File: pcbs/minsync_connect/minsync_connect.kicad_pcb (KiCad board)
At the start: 2 copper layers, 17.4 x 14 mm, 2 parts, among them J1 Left, J2 Right

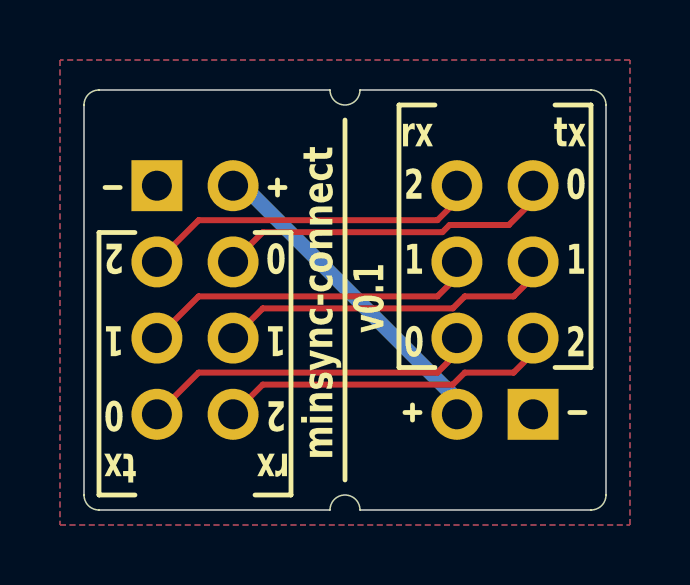
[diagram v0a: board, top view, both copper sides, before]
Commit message: Order minsync
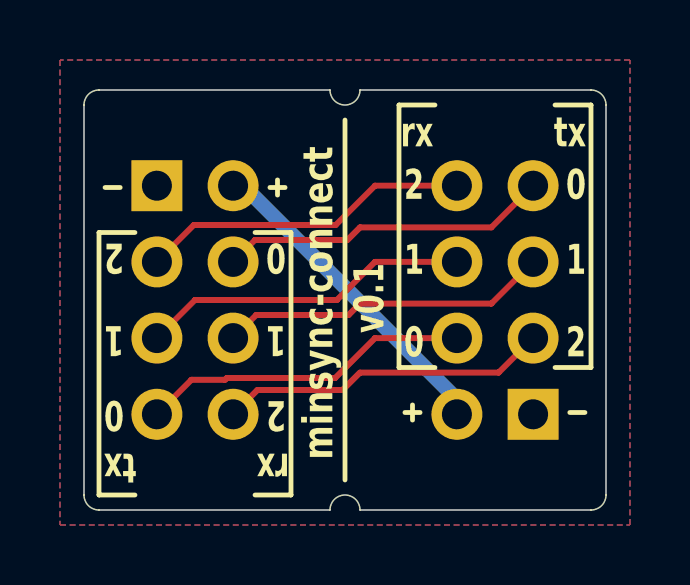
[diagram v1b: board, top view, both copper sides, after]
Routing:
- net /L_TX2: track 11.6 -> 11.1 mm
- net /L_TX0: track 11.6 -> 11.1 mm
- net /L_RX2: track 11.6 -> 11.1 mm
- net /L_RX0: track 11.6 -> 11.1 mm
- net /L_TX1: track 11.6 -> 11.1 mm
- net /L_RX1: track 11.6 -> 11.1 mm
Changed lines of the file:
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@@
 	)
 	(segment
-		(start 152.26 42.82)
-		(end 158.593654 42.82)
+		(start 155.5 42.42)
+		(end 160.12 42.42)
+		(width 0.2)
+		(layer "F.Cu")
+		(net 1)
+	)
+	(segment
+		(start 160.12 42.42)
+		(end 161.27 41.27)
+		(width 0.2)
+		(layer "F.Cu")
+		(net 1)
+	)
+	(segment
+		(start 154.92 43)
+		(end 155.5 42.42)
 		(width 0.2)
 		(layer "F.Cu")
@@
 	(segment
 		(start 151.27 43.81)
-		(end 152.26 42.82)
-		(width 0.2)
-		(layer "F.Cu")
-		(net 1)
-	)
-	(segment
-		(start 160.62 42.42)
-		(end 161.77 41.27)
-		(width 0.2)
-		(layer "F.Cu")
-		(net 1)
-	)
-	(segment
-		(start 158.593654 42.82)
-		(end 158.993654 42.42)
-		(width 0.2)
-		(layer "F.Cu")
-		(net 1)
-	)
-	(segment
-		(start 158.993654 42.42)
-		(end 160.62 42.42)
+		(end 152.08 43)
+		(width 0.2)
+		(layer "F.Cu")
+		(net 1)
+	)
+	(segment
+		(start 152.08 43)
+		(end 154.92 43)
 		(width 0.2)
 		(layer "F.Cu")
@@
 	(segment
 		(start 148.73 41.27)
-		(end 150.12 39.88)
-		(width 0.2)
-		(layer "F.Cu")
-		(net 2)
-	)
-	(segment
-		(start 150.12 39.88)
-		(end 158.08 39.88)
-		(width 0.2)
-		(layer "F.Cu")
-		(net 2)
-	)
-	(segment
-		(start 158.08 39.88)
-		(end 159.23 38.73)
-		(width 0.2)
-		(layer "F.Cu")
-		(net 2)
-	)
-	(segment
-		(start 158.593654 40.28)
-		(end 158.993654 39.88)
-		(width 0.2)
-		(layer "F.Cu")
-		(net 3)
-	)
-	(segment
-		(start 160.62 39.88)
-		(end 161.77 38.73)
-		(width 0.2)
-		(layer "F.Cu")
-		(net 3)
-	)
-	(segment
-		(start 158.993654 39.88)
-		(end 160.62 39.88)
-		(width 0.2)
-		(layer "F.Cu")
-		(net 3)
+		(end 150 40)
+		(width 0.2)
+		(layer "F.Cu")
+		(net 2)
+	)
+	(segment
+		(start 150 40)
+		(end 154.73 40)
+		(width 0.2)
+		(layer "F.Cu")
+		(net 2)
+	)
+	(segment
+		(start 154.73 40)
+		(end 156 38.73)
+		(width 0.2)
+		(layer "F.Cu")
+		(net 2)
+	)
+	(segment
+		(start 156 38.73)
+		(end 158.73 38.73)
+		(width 0.2)
+		(layer "F.Cu")
+		(net 2)
 	)
 	(segment
 		(start 151.27 41.27)
-		(end 152.26 40.28)
-		(width 0.2)
-		(layer "F.Cu")
-		(net 3)
-	)
-	(segment
-		(start 152.26 40.28)
-		(end 158.593654 40.28)
-		(width 0.2)
-		(layer "F.Cu")
-		(net 3)
+		(end 152.04 40.5)
+		(width 0.2)
+		(layer "F.Cu")
+		(net 3)
+	)
+	(segment
+		(start 152.04 40.5)
+		(end 155.12 40.5)
+		(width 0.2)
+		(layer "F.Cu")
+		(net 3)
+	)
+	(segment
+		(start 159.88 40.12)
+		(end 161.27 38.73)
+		(width 0.2)
+		(layer "F.Cu")
+		(net 3)
+	)
+	(segment
+		(start 155.5 40.12)
+		(end 159.88 40.12)
+		(width 0.2)
+		(layer "F.Cu")
+		(net 3)
+	)
+	(segment
+		(start 155.12 40.5)
+		(end 155.5 40.12)
+		(width 0.2)
+		(layer "F.Cu")
+		(net 3)
+	)
+	(segment
+		(start 156 36.19)
+		(end 158.73 36.19)
+		(width 0.2)
+		(layer "F.Cu")
+		(net 4)
+	)
+	(segment
+		(start 149.96 37.5)
+		(end 154.69 37.5)
+		(width 0.2)
+		(layer "F.Cu")
+		(net 4)
+	)
+	(segment
+		(start 154.69 37.5)
+		(end 156 36.19)
+		(width 0.2)
+		(layer "F.Cu")
+		(net 4)
 	)
 	(segment
 		(start 148.73 38.73)
-		(end 150.12 37.34)
-		(width 0.2)
-		(layer "F.Cu")
-		(net 4)
-	)
-	(segment
-		(start 158.08 37.34)
-		(end 159.23 36.19)
-		(width 0.2)
-		(layer "F.Cu")
-		(net 4)
-	)
-	(segment
-		(start 150.12 37.34)
-		(end 158.08 37.34)
-		(width 0.2)
-		(layer "F.Cu")
-		(net 4)
+		(end 149.96 37.5)
+		(width 0.2)
+		(layer "F.Cu")
+		(net 4)
+	)
+	(segment
+		(start 154.67 42.6)
+		(end 156 41.27)
+		(width 0.2)
+		(layer "F.Cu")
+		(net 5)
 	)
 	(segment
 		(start 148.73 43.81)
-		(end 150.12 42.42)
-		(width 0.2)
-		(layer "F.Cu")
-		(net 5)
-	)
-	(segment
-		(start 158.08 42.42)
-		(end 159.23 41.27)
-		(width 0.2)
-		(layer "F.Cu")
-		(net 5)
-	)
-	(segment
-		(start 150.12 42.42)
-		(end 158.08 42.42)
-		(width 0.2)
-		(layer "F.Cu")
-		(net 5)
-	)
-	(segment
-		(start 161.77 36.19)
-		(end 160.46 37.5)
-		(width 0.2)
-		(layer "F.Cu")
-		(net 6)
-	)
-	(segment
-		(start 160.46 37.5)
-		(end 158.485686 37.5)
-		(width 0.2)
-		(layer "F.Cu")
-		(net 6)
-	)
-	(segment
-		(start 158.245686 37.74)
-		(end 152.26 37.74)
-		(width 0.2)
-		(layer "F.Cu")
-		(net 6)
-	)
-	(segment
-		(start 152.26 37.74)
-		(end 151.27 38.73)
-		(width 0.2)
-		(layer "F.Cu")
-		(net 6)
-	)
-	(segment
-		(start 158.485686 37.5)
-		(end 158.245686 37.74)
-		(width 0.2)
-		(layer "F.Cu")
+		(end 149.88 42.66)
+		(width 0.2)
+		(layer "F.Cu")
+		(net 5)
+	)
+	(segment
+		(start 151 42.66)
+		(end 151.06 42.6)
+		(width 0.2)
+		(layer "F.Cu")
+		(net 5)
+	)
+	(segment
+		(start 149.88 42.66)
+		(end 151 42.66)
+		(width 0.2)
+		(layer "F.Cu")
+		(net 5)
+	)
+	(segment
+		(start 151.06 42.6)
+		(end 154.67 42.6)
+		(width 0.2)
+		(layer "F.Cu")
+		(net 5)
+	)
+	(segment
+		(start 156 41.27)
+		(end 158.73 41.27)
+		(width 0.2)
+		(layer "F.Cu")
+		(net 5)
+	)
+	(segment
+		(start 155.08 38)
+		(end 155.5 37.58)
+		(width 0.2)
+		(layer "F.Cu")
+		(net 6)
+	)
+	(segment
+		(start 151.27 38.73)
+		(end 152 38)
+		(width 0.2)
+		(layer "F.Cu")
+		(net 6)
+	)
+	(segment
+		(start 155.5 37.58)
+		(end 159.88 37.58)
+		(width 0.2)
+		(layer "F.Cu")
+		(net 6)
+	)
+	(segment
+		(start 159.88 37.58)
+		(end 161.27 36.19)
+		(width 0.2)
+		(layer "F.Cu")
+		(net 6)
+	)
+	(segment
+		(start 152 38)
+		(end 155.08 38)
+		(width 0.2)
+		(layer "F.Cu")
